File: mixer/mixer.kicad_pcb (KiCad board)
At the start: 4 copper layers, 182.9 x 153.8 mm, 99 parts, among them J1 EURORACK_CONN_16, J10 C_BOARD_IN, J11 INTERCONNECT1, J12 M_BOARD_IN, J13 INTERCONNECT2, J14 C_BOARD_OUT, J15 C_IN1, J16 C_IN2, J17 C_AUXSEND1, J18 C_PAN1, J19 C_AUXSEND2, J2 AUX_OUT, J20 C_PAN2, J21 M_OUT_L, J22 M_AUXSEND, J23 M_AUX_AMOUNT, J24 M_OUT_R, J25 M_AUX_RETURN_L, J26 M_AUX_RETURN_L, J27 M_MASTER, J3 AUX_IN_R, J4 AUX_IN_L, J5 MAIN_OUT_R, J6 MAIN_OUT_L, J7 CHANNEL_IN, J8 AVR-ISP-6, J9 CHANNEL_IN, Q1 BSS214NW, SW1 MUTE_PBSW, SW2 SOLO_PBSW, SW3 AUX_PRE_POST_FADER_SLIDESW, SW4 MUTE_PBSW, SW5 SOLO_PBSW, SW6 AUX_PRE_POST_FADER_SLIDESW, U1 TL074, U2 TL074, U3 DG403, U4 TL074, U6 ATtiny24-20SS

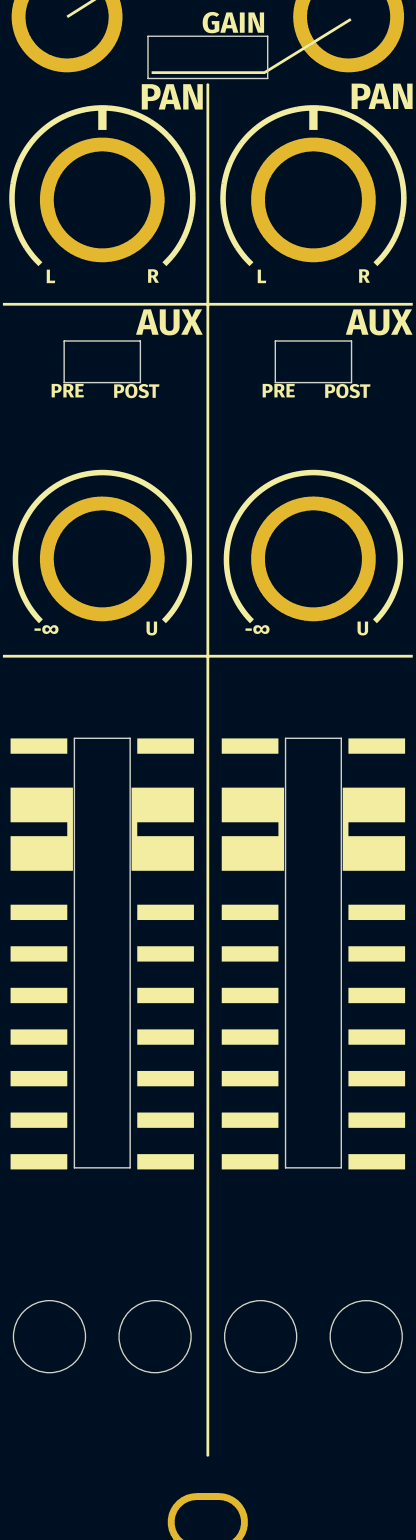
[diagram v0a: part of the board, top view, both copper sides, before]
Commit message: update todos
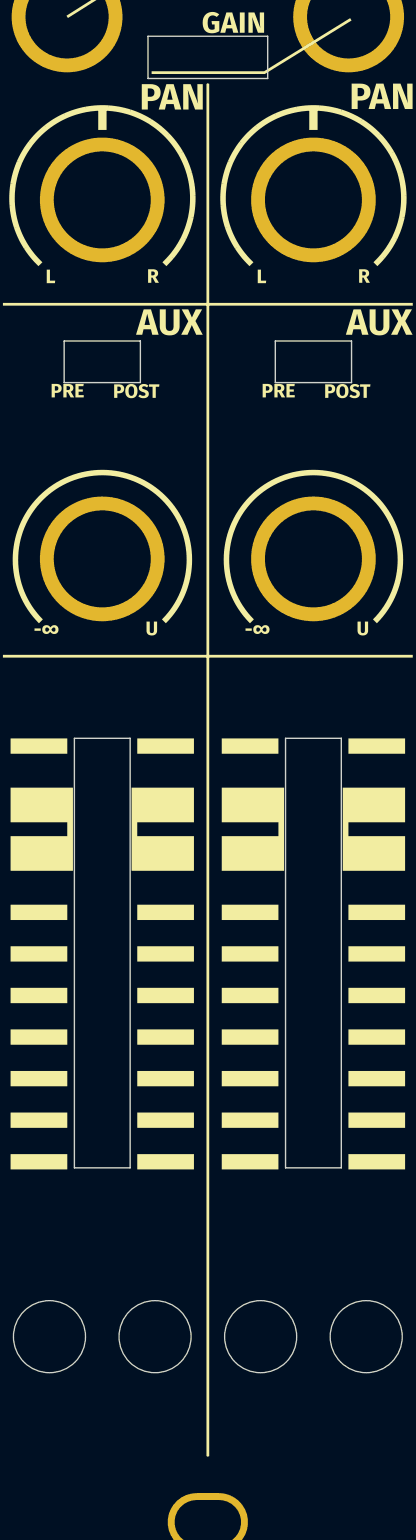
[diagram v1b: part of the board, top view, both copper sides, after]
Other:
- board text added: "TODO: aux return should have gain"
- board text added: "TODO: switch back to M + S"
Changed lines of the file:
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@@
 		(end 40.639375 161.278221)
 		(stroke
-			(width 0)
+			(width 0.1)
 			(type solid)
 		)
@@
 		)
 	)
+	(gr_text "TODO: switch back to M + S"
+		(at 237.871 101.219 0)
+		(layer "User.1")
+		(effects
+			(font
+				(size 1 1)
+				(thickness 0.15)
+			)
+			(justify left bottom)
+		)
+	)
 	(gr_text "TODO: confirm all cutout sizes"
 		(at 234.95 66.548 0)
@@
 		(layer "User.1")
 		(effects
+			(font
+				(size 1 1)
+				(thickness 0.15)
+			)
+			(justify left bottom)
+		)
+	)
+	(gr_text "TODO: aux return should have gain"
+		(at 241.681 95.123 0)
+		(layer "User.1")
+		(effects
